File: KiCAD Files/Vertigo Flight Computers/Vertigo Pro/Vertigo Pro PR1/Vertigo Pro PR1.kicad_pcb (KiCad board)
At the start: 4 copper layers, 45.2 x 81.8 mm, 151 parts, among them IC1 ICM-20602, IC2 DPS310XTSA1, J1 ST-LINK Conn, J2 USB_C_2.0, J3 FFC2A32-24-T, J4 Screw_Terminal, J5 Screw_Terminal, J6 Screw_Terminal, J7 Screw_Terminal, Q1 MMBT3904-TP, Q2 MMBT3904-TP, Q3 FDN339AN, Q4 FDN339AN, Q5 SI7149ADP-T1-GE3, Q6 MMBT3904-TP, Q7 MMBT3904-TP, Q8 FDN339AN, Q9 FDN339AN, SW1 SW_SPDT, U1 STM32F103C8Tx, U10 TPS79133DBVR, U12 TLV709, U13 TLV75528PDBV, U2 AP63203WU, U3 ESP32-S3-WROOM-1, U4 TLV75515PDBV, U5 TLV709, U8 NEO-6M-GPS, U9 24AA32A-I_MS, Y1 16MHz

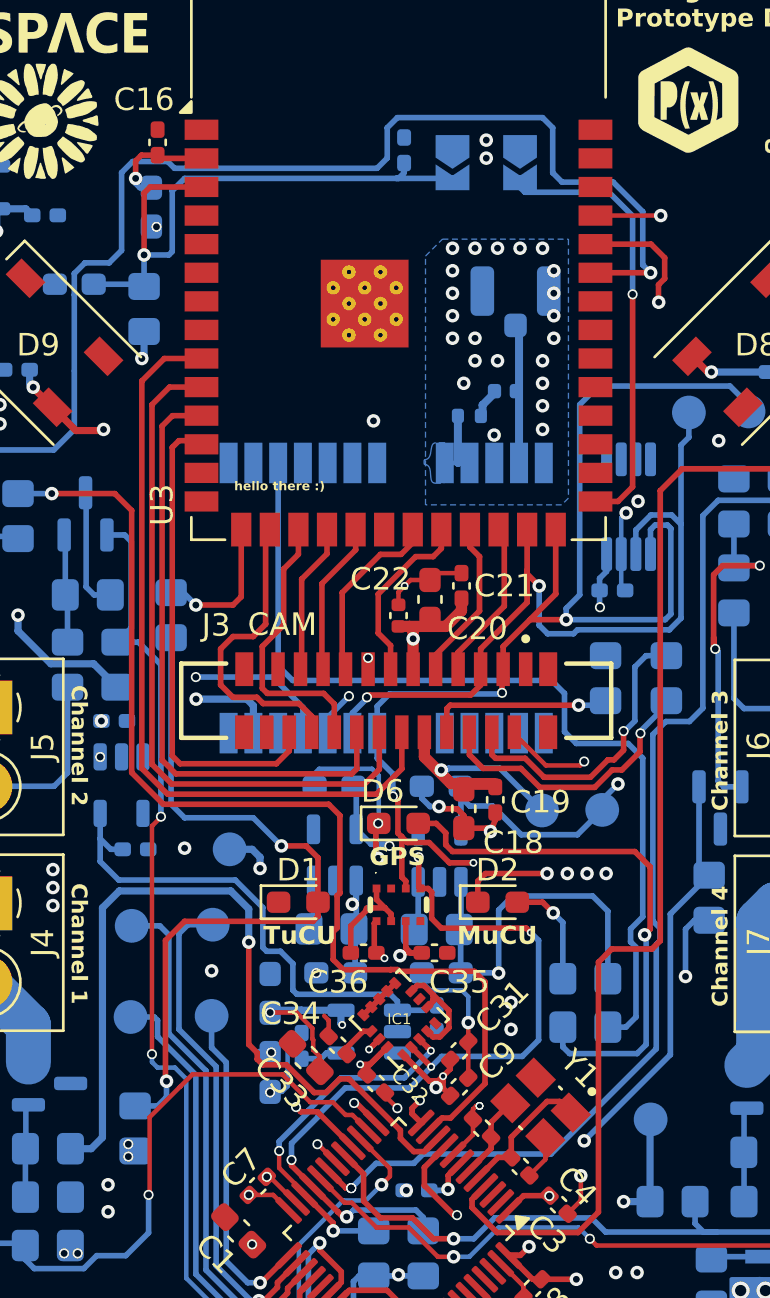
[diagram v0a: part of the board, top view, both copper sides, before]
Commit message: Via fix, est
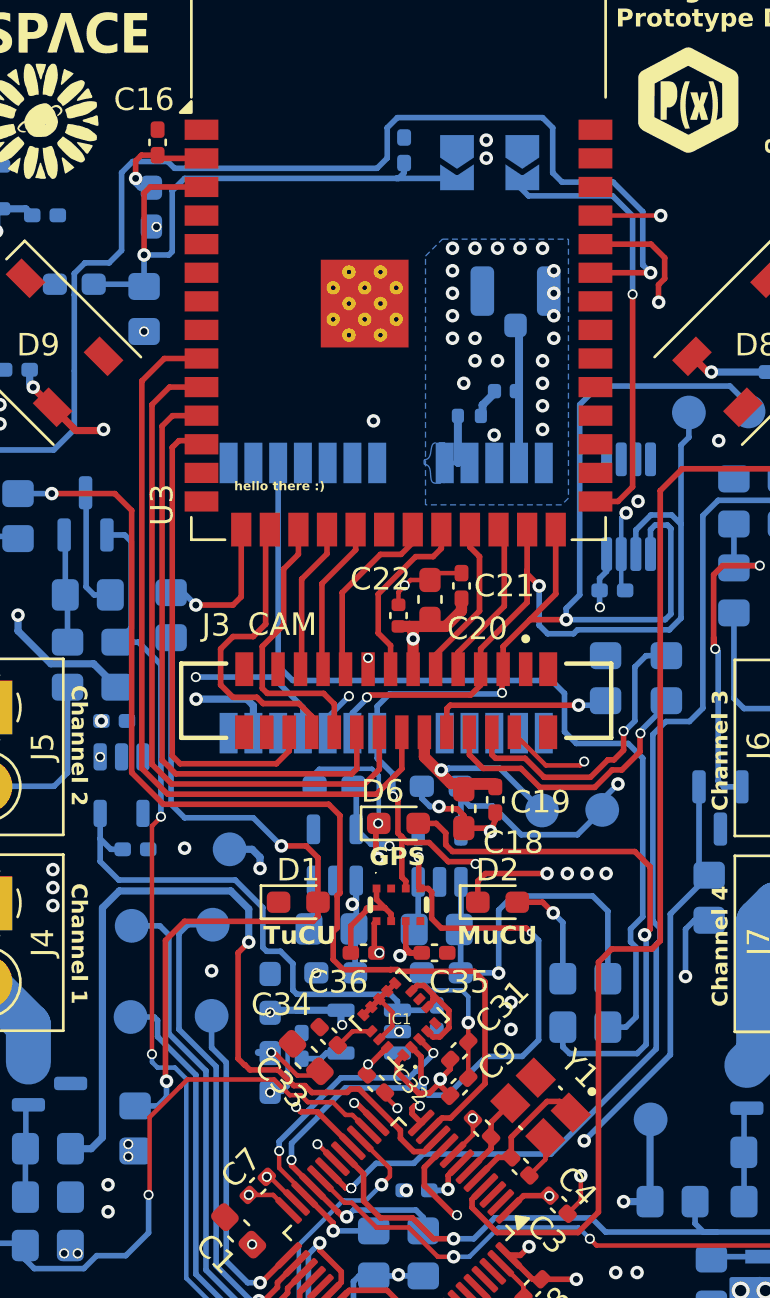
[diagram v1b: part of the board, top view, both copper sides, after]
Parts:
- removed BOOT, RST: Jumper_2_Open, Jumper:SolderJumper-2_P1.3mm_Open_TrianglePad1.0x1.5mm
- added JP1: Jumper_2_Open, Jumper:SolderJumper-2_P1.3mm_Open_TrianglePad1.0x1.5mm, B.Cu at (151.2, 78.2)
- added JP2: Jumper_2_Open, Jumper:SolderJumper-2_P1.3mm_Open_TrianglePad1.0x1.5mm, B.Cu at (154.1, 78.2)
- moved C34 0.57 mm to (145.5, 117.0)
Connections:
- AE1 pad 2: AGND -> (no net)
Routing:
- net /ULN_3V3: track 34.0 -> 30.8 mm
- net /STM_UART2_TX: track 39.2 -> 36.1 mm
- net +3.3V: track 109.3 -> 107.1 mm, vias 54 -> 53
- net /ESP_I2C_SCL: track 84.3 -> 85.5 mm
- net /ESP_I2C_SDA: track 82.5 -> 83.3 mm
- net AGND: track 80.6 -> 80.5 mm, vias 95 -> 94
